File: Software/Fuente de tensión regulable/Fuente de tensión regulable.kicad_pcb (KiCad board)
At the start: 2 copper layers, 79 x 65 mm, 34 parts, among them J2 conector DC, J3 conector current, SW1 SW_Wuerth_450301014042, U1 L7805, U3 LM2596S-12

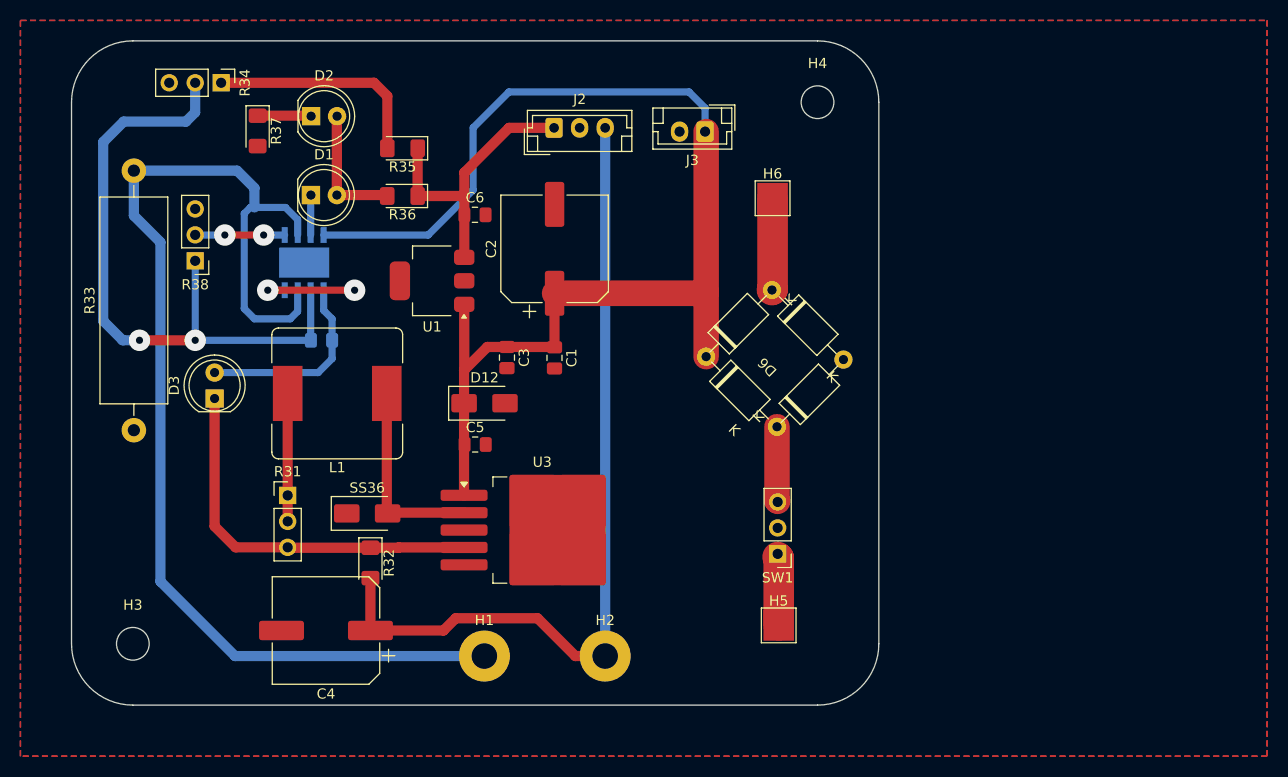
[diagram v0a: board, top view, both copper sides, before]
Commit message: Add files via upload
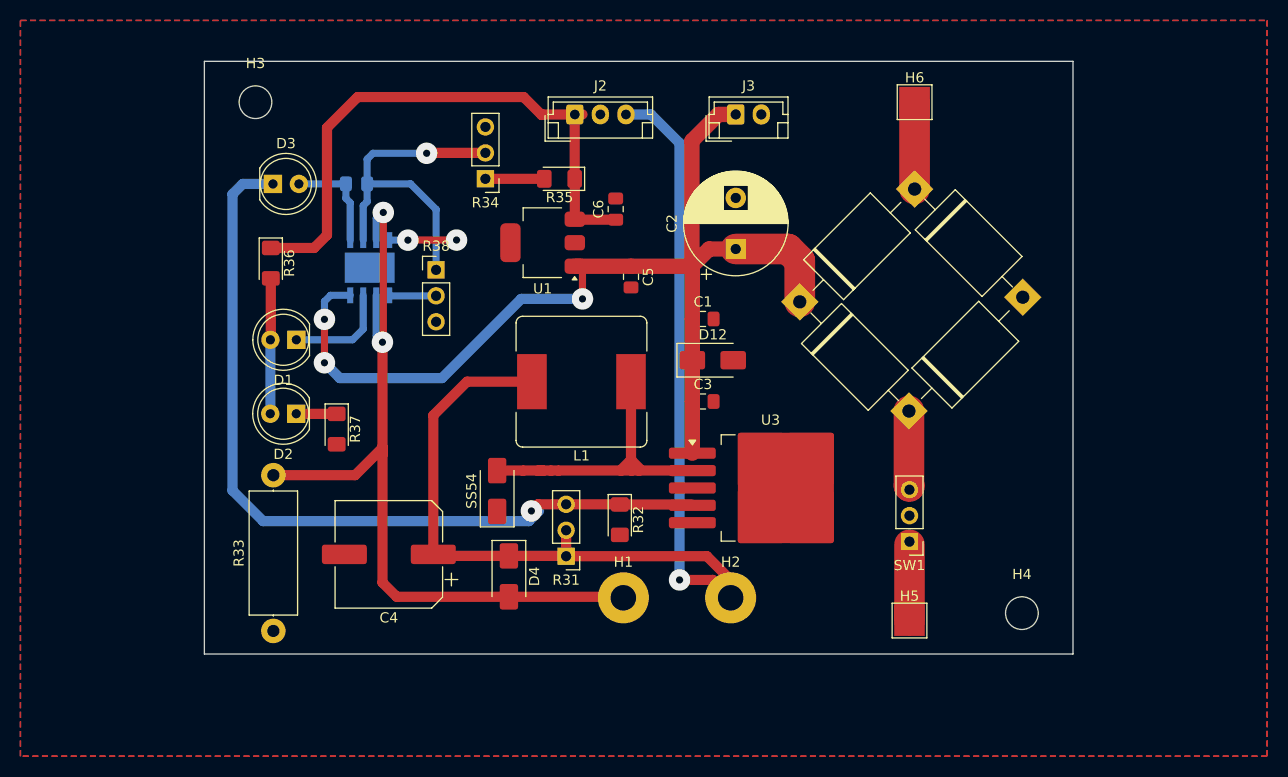
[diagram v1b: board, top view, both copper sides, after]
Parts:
- removed SS36: D_Schottky_Dual_CommonAnode_AKK_Split, Diode_SMD:D_SMA
- added D4: 1N4007, Diode_SMD:D_SMA, F.Cu at (164.8, 101.4)
- added SS54: D_Schottky_Dual_CommonAnode_AKK_Split, Diode_SMD:D_SMA, F.Cu at (163.7, 93.0)
- C2: footprint Capacitor_SMD:CP_Elec_10x7.9 -> Capacitor_THT:CP_Radial_D10.0mm_P5.00mm
- R33: value 0.2-2W -> 0.2-5W; footprint Resistor_THT:R_Axial_Power_L20.0mm_W6.4mm_P25.40mm -> Resistor_THT:R_Axial_DIN0414_L11.9mm_D4.5mm_P15.24mm_Horizontal
- moved H3 54.3 mm to (140.0, 55.0)
- moved H4 53.9 mm to (215.0, 105.0)
- moved R37 30.2 mm to (147.9, 87.0)
- moved D2 29.2 mm to (144.0, 85.5), turned to 180 degrees
- moved R31 27.9 mm to (170.4, 99.4), turned to 180 degrees
- moved R34 27.5 mm to (162.5, 62.5), turned to 180 degrees
- moved R32 24.8 mm to (175.7, 95.8)
- moved L1 23.9 mm to (171.9, 82.3)
- moved R33 23.9 mm to (141.8, 106.7)
- moved R38 23.6 mm to (157.7, 71.4), turned to 0 degrees
- moved D12 22.7 mm to (184.8, 80.2)
- moved U3 22.7 mm to (190.4, 92.8)
- moved C5 22.4 mm to (176.8, 72.1), turned to -90 degrees
- moved D3 21.8 mm to (141.7, 63.0), turned to 0 degrees
- moved C3 19.7 mm to (183.8, 84.3), turned to 0 degrees
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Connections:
- L1 pad 2: Net-(L1-Pad2) -> /Vout+
- R31 pad 1: Net-(L1-Pad2) -> /Vout+
- R31 pad 2: Net-(L1-Pad2) -> /Vout+
- R32 pad 2: /Vout+ -> GND
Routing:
- net Net-(D3-K): track 37.8 -> 81.0 mm, vias 0 -> 1
- net /Vout-: track 115.2 -> 81.4 mm, vias 0 -> 2
- net /Vout+: track 81.8 -> 113.8 mm, vias 0 -> 1
- net Net-(A8A--): track 64.4 -> 33.6 mm, vias 2 -> 1
- net 5v: track 28.2 -> 57.8 mm
- net /+: track 120.5 -> 104.3 mm, vias 0 -> 3
- net Net-(R34-Pad1): track 21.9 -> 5.76 mm
- net Net-(L1-Pad2): track 12.5 -> 0.00 mm
- net Net-(SS54A-K): track 19.4 -> 30.8 mm
- net Net-(D3-A): track 19.1 -> 10.3 mm
- net Net-(D1-K): track 3.98 -> 10.3 mm
- net Net-(A8B-+): track 8.77 -> 4.61 mm, vias 2 -> 0
- net GND: track 10.2 -> 6.61 mm
- net Net-(D2-K): track 5.26 -> 3.97 mm
- net Net-(SW1-B): track 6.73 -> 7.41 mm
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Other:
- board size 79 x 65 mm -> 85 x 58 mm
